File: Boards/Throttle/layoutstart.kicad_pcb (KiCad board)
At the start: 2 copper layers, 59.7 x 53.5 mm, 70 parts, among them J1 micromatch_female_TOP_ENTRY_l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, J2 micromatch_female_TOP_ENTRY_l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, J3 CONN_02X03, Q1 SSM3K333R, Q2 SSM3K333R, Q3 SSM3K333R, Q4 SSM3K333R, U1 MCP6001, U2 TPS561201, U3 MCP6001, U4 CAN_Transceiver, Y1 Crystal_SMD

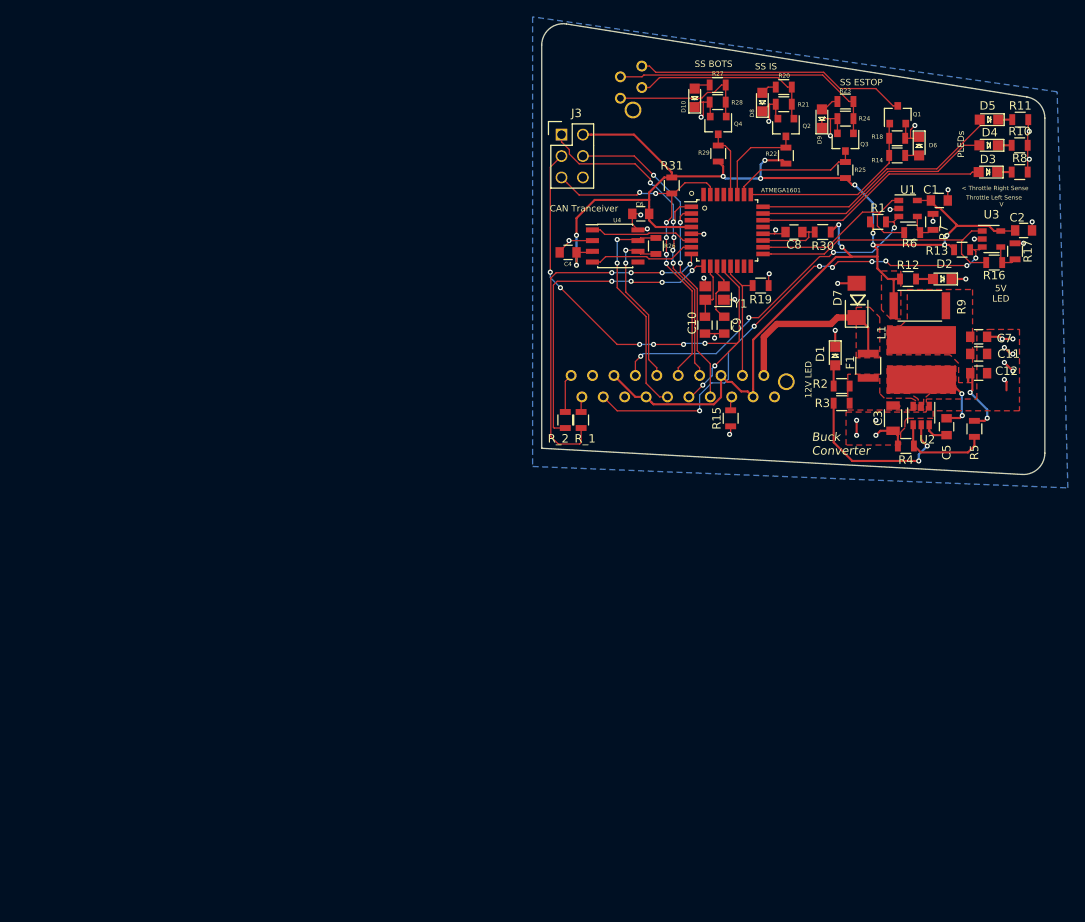
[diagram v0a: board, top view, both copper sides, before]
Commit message: Finished REV2 layout
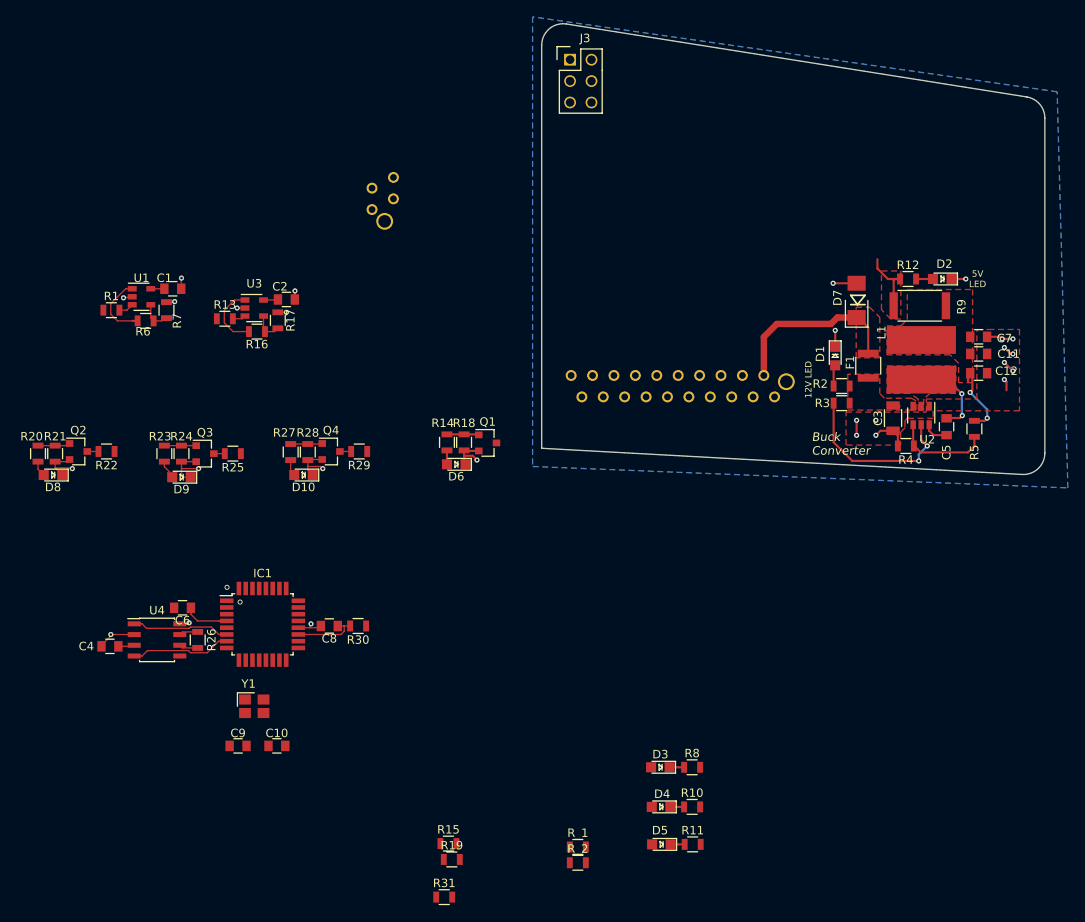
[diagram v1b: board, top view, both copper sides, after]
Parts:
- moved R20 98.6 mm to (36.6, 95.0), turned to 270 degrees
- moved R21 95.9 mm to (38.6, 95.0), turned to 270 degrees
- moved D8 95.1 mm to (38.4, 97.5), turned to 180 degrees
- moved D5 94.4 mm to (110.5, 141.4)
- moved R11 94.4 mm to (114.2, 141.4)
- moved Q2 92.3 mm to (41.4, 94.7), turned to 0 degrees
- moved R1 91.5 mm to (45.3, 78.0)
- moved C1 91.5 mm to (52.6, 75.4)
- moved R6 91.5 mm to (49.3, 79.2)
- moved R7 91.5 mm to (51.8, 78.0)
- moved U1 91.5 mm to (48.9, 76.4)
- moved R23 91.0 mm to (51.6, 95.0), turned to 270 degrees
- moved R31 88.6 mm to (84.8, 147.6), turned to 0 degrees
- moved R24 88.2 mm to (53.6, 95.0), turned to 270 degrees
- moved R22 87.9 mm to (44.7, 94.7), turned to 180 degrees
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- renumbered ATMEGA1601 to IC1
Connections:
- IC1 pad 26: /SS_EStop_Out_n -> /SS_Inertia_Out_n
- IC1 pad 27: /SS_Inertia_Out_n -> /SS_BOTS_Out_n
- IC1 pad 28: /SS_BOTS_Out_n -> /SS_EStop_Out_n
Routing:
- net VCC: track 171.6 -> 18.8 mm, vias 12 -> 0
- net /SCK: track 59.4 -> 0.00 mm, vias 8 -> 0
- net /Throttle2_Left_Sense: track 58.5 -> 1.57 mm, vias 8 -> 0
- net /RESET: track 44.2 -> 0.00 mm, vias 6 -> 0
- net Net-(IC1-Pad8): track 43.0 -> 0.00 mm, vias 4 -> 0
- net /Throttle1_Right_Sense: track 44.5 -> 1.54 mm, vias 4 -> 0
- net /MISO: track 42.9 -> 0.00 mm, vias 5 -> 0
- net /MOSI: track 40.6 -> 0.00 mm, vias 3 -> 0
- net Net-(IC1-Pad9): track 37.2 -> 0.00 mm, vias 4 -> 0
- net /RTD: track 32.3 -> 0.00 mm
- net /ProgrammingLED3: track 30.4 -> 0.00 mm
- net /SS_Cockpit_EStop: track 32.8 -> 3.78 mm
- net /ProgrammingLED2: track 29.0 -> 0.00 mm
- net /ProgrammingLED1: track 28.0 -> 0.00 mm
- net /Throttle1Adjusted: track 32.2 -> 7.81 mm
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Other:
- board text removed: "< Throttle Right Sense"
- board text removed: "CAN Tranceiver"
- board text removed: "PLEDs"
- board text removed: "SS BOTS"
- board text removed: "SS ESTOP"
- board text removed: "SS IS"
- board text removed: "Throttle Left Sense V"
